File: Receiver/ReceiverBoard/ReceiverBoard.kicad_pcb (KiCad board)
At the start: 2 copper layers, 100 x 120 mm, 50 parts, among them IC1 SN74HCT245PWR, IC2 SN74HCT245PWR, J1 Left Header, J10 Output 5, J11 Output 6, J12 Output 7, J13 High Power, J14 Output 8, J15 Output 9, J16 Output 10, J17 Output 11, J18 Output 12, J19 Output 13, J2 Right Header, J20 Output 14, J21 Output 15, J22 J1B1211CCD, J3 Upper Middle Header, J4 Lower Middle Header, J5 Output 0, J6 Output 1, J7 Output 2, J8 Output 3, J9 Output 4

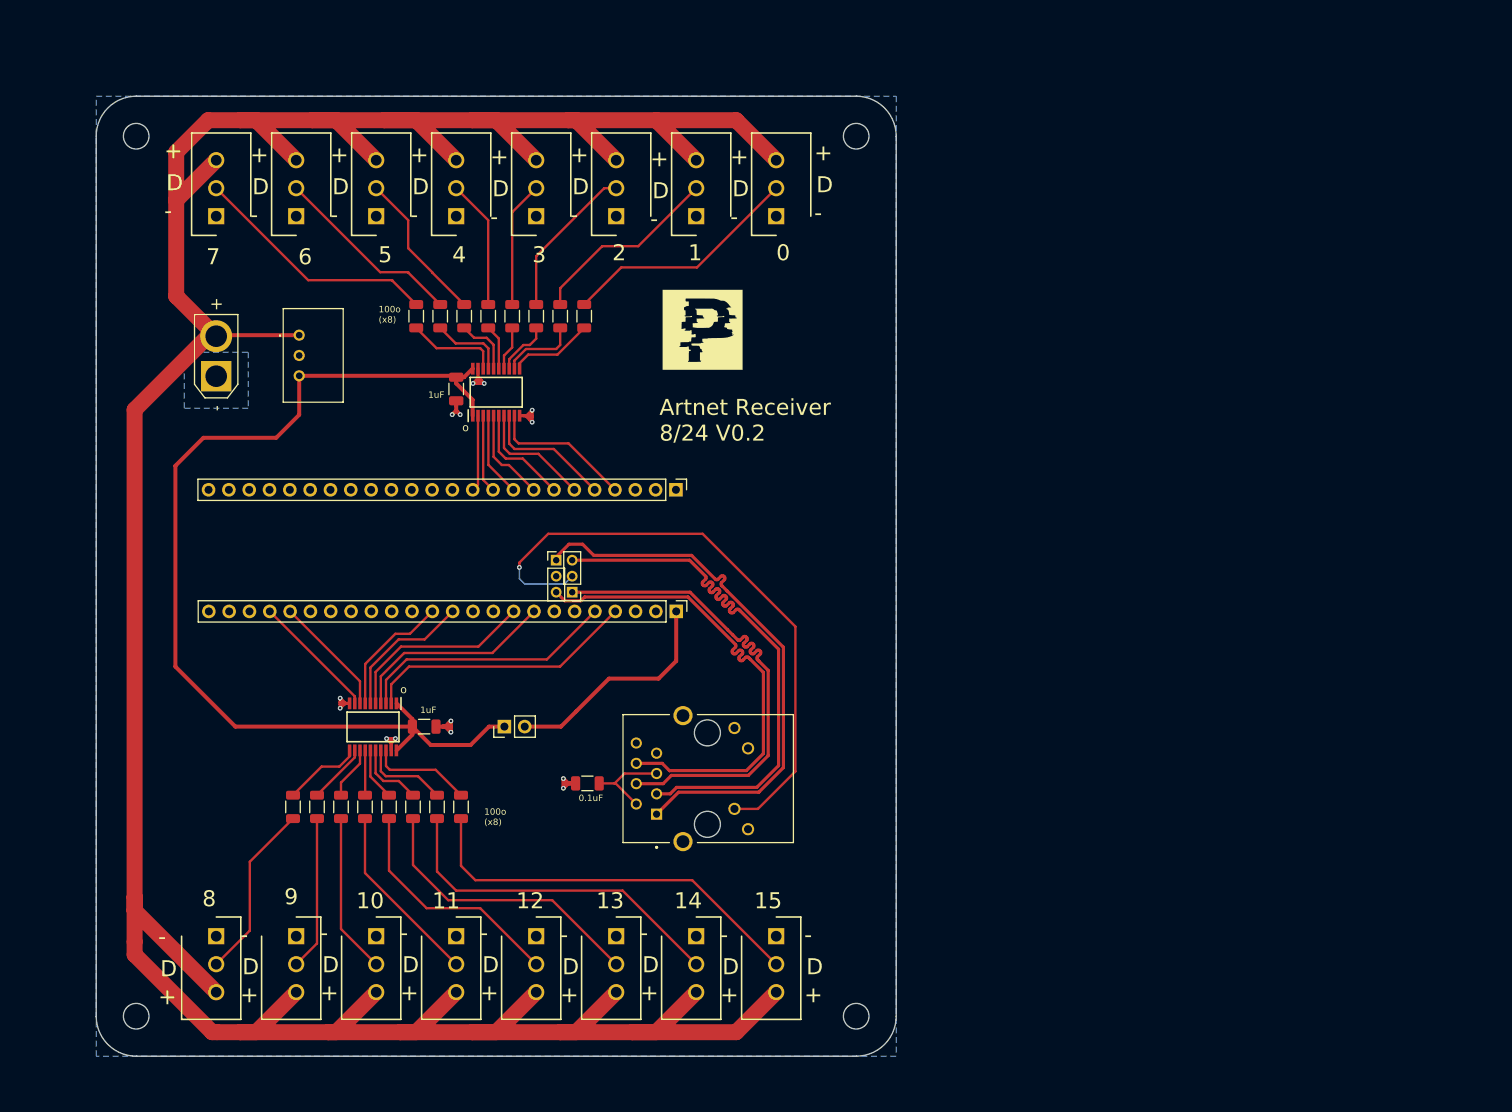
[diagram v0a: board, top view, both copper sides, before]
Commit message: Artnet is up and running!
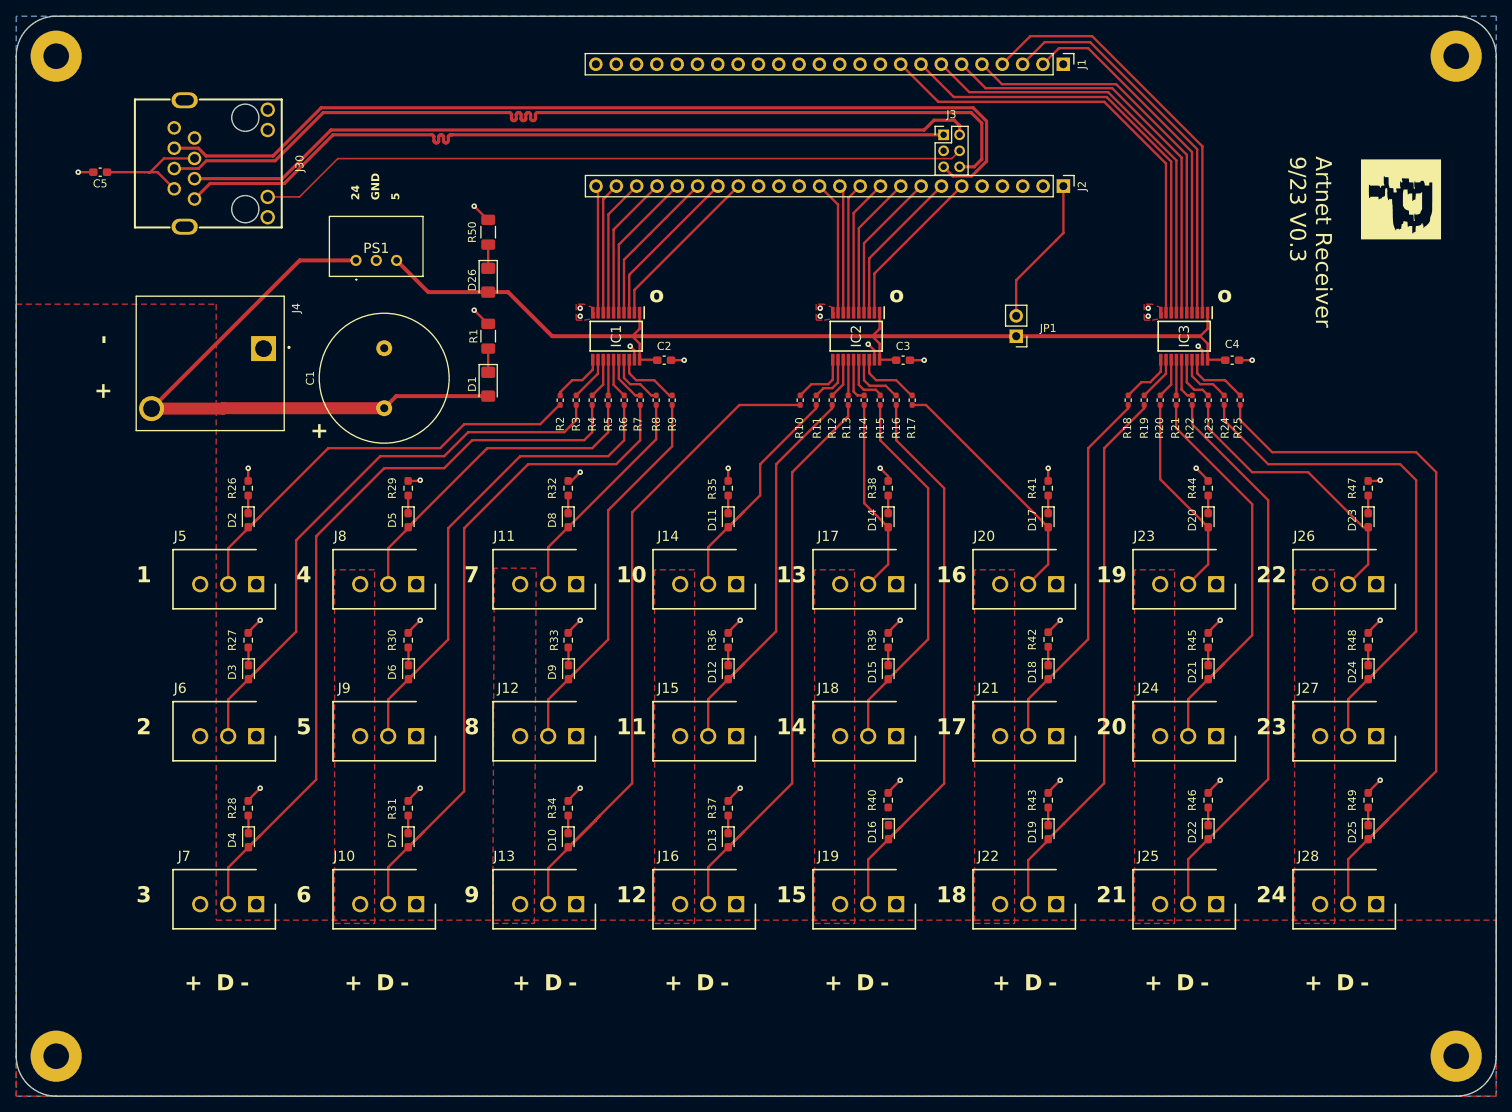
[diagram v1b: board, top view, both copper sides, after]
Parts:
- added C4: 1u, Capacitor_SMD:C_0603_1608Metric_Pad1.08x0.95mm_HandSolder, F.Cu at (217.0, 68.0)
- added C5: 100n, Capacitor_SMD:C_0603_1608Metric_Pad1.08x0.95mm_HandSolder, F.Cu at (75.5, 44.5)
- added D1: RED, LED_SMD:LED_1206_3216Metric_Pad1.42x1.75mm_HandSolder, F.Cu at (124.0, 71.0)
- added D10: YELLOW, LED_SMD:LED_0603_1608Metric_Pad1.05x0.95mm_HandSolder, F.Cu at (134.0, 128.0)
- added D11: YELLOW, LED_SMD:LED_0603_1608Metric_Pad1.05x0.95mm_HandSolder, F.Cu at (154.0, 88.0)
- added D12: YELLOW, LED_SMD:LED_0603_1608Metric_Pad1.05x0.95mm_HandSolder, F.Cu at (154.0, 107.0)
- added D13: YELLOW, LED_SMD:LED_0603_1608Metric_Pad1.05x0.95mm_HandSolder, F.Cu at (154.0, 128.0)
- added D14: YELLOW, LED_SMD:LED_0603_1608Metric_Pad1.05x0.95mm_HandSolder, F.Cu at (174.0, 88.0)
- added D15: YELLOW, LED_SMD:LED_0603_1608Metric_Pad1.05x0.95mm_HandSolder, F.Cu at (174.0, 107.0)
- added D16: YELLOW, LED_SMD:LED_0603_1608Metric_Pad1.05x0.95mm_HandSolder, F.Cu at (174.0, 127.0)
- added D17: YELLOW, LED_SMD:LED_0603_1608Metric_Pad1.05x0.95mm_HandSolder, F.Cu at (194.0, 88.0)
- added D18: YELLOW, LED_SMD:LED_0603_1608Metric_Pad1.05x0.95mm_HandSolder, F.Cu at (194.0, 107.0)
- added D19: YELLOW, LED_SMD:LED_0603_1608Metric_Pad1.05x0.95mm_HandSolder, F.Cu at (194.0, 127.0)
- added D2: YELLOW, LED_SMD:LED_0603_1608Metric_Pad1.05x0.95mm_HandSolder, F.Cu at (94.0, 88.0)
- added D20: YELLOW, LED_SMD:LED_0603_1608Metric_Pad1.05x0.95mm_HandSolder, F.Cu at (214.0, 88.0)
- added D21: YELLOW, LED_SMD:LED_0603_1608Metric_Pad1.05x0.95mm_HandSolder, F.Cu at (214.0, 107.0)
- added D22: YELLOW, LED_SMD:LED_0603_1608Metric_Pad1.05x0.95mm_HandSolder, F.Cu at (214.0, 127.0)
- added D23: YELLOW, LED_SMD:LED_0603_1608Metric_Pad1.05x0.95mm_HandSolder, F.Cu at (234.0, 88.0)
- added D24: YELLOW, LED_SMD:LED_0603_1608Metric_Pad1.05x0.95mm_HandSolder, F.Cu at (234.0, 107.0)
- added D25: YELLOW, LED_SMD:LED_0603_1608Metric_Pad1.05x0.95mm_HandSolder, F.Cu at (234.0, 127.0)
- added D26: RED, LED_SMD:LED_1206_3216Metric_Pad1.42x1.75mm_HandSolder, F.Cu at (124.0, 58.0)
- added D3: YELLOW, LED_SMD:LED_0603_1608Metric_Pad1.05x0.95mm_HandSolder, F.Cu at (94.0, 107.0)
- added D4: YELLOW, LED_SMD:LED_0603_1608Metric_Pad1.05x0.95mm_HandSolder, F.Cu at (94.0, 128.0)
- added D5: YELLOW, LED_SMD:LED_0603_1608Metric_Pad1.05x0.95mm_HandSolder, F.Cu at (114.0, 88.0)
- added D6: YELLOW, LED_SMD:LED_0603_1608Metric_Pad1.05x0.95mm_HandSolder, F.Cu at (114.0, 107.0)
- added D7: YELLOW, LED_SMD:LED_0603_1608Metric_Pad1.05x0.95mm_HandSolder, F.Cu at (114.0, 128.0)
- added D8: YELLOW, LED_SMD:LED_0603_1608Metric_Pad1.05x0.95mm_HandSolder, F.Cu at (134.0, 88.0)
- added D9: YELLOW, LED_SMD:LED_0603_1608Metric_Pad1.05x0.95mm_HandSolder, F.Cu at (134.0, 107.0)
- added IC3: SN74HCT245PWR, SN74HCT245PWR:SOP65P640X120-20N, F.Cu at (211.0, 65.0)
- added J23: String, 284514-3:SHDR3W80P0X350_1X3_1250X725X940P, F.Cu at (215.0, 96.0)
- added J24: String, 284514-3:SHDR3W80P0X350_1X3_1250X725X940P, F.Cu at (215.0, 115.0)
- added J25: String, 284514-3:SHDR3W80P0X350_1X3_1250X725X940P, F.Cu at (215.0, 136.0)
- added J26: String, 284514-3:SHDR3W80P0X350_1X3_1250X725X940P, F.Cu at (235.0, 96.0)
- added J27: String, 284514-3:SHDR3W80P0X350_1X3_1250X725X940P, F.Cu at (235.0, 115.0)
- added J28: String, 284514-3:SHDR3W80P0X350_1X3_1250X725X940P, F.Cu at (235.0, 136.0)
- added J30: RVB-ZZ-0004, RVB-ZZ-0004:RJ45-TH_RVB-ZZ-0004, F.Cu at (90.6, 43.4)
- added R17: 100, Resistor_SMD:R_0402_1005Metric_Pad0.72x0.64mm_HandSolder, F.Cu at (177.0, 73.0)
- added R18: 100, Resistor_SMD:R_0402_1005Metric_Pad0.72x0.64mm_HandSolder, F.Cu at (204.0, 73.0)
- added R19: 100, Resistor_SMD:R_0402_1005Metric_Pad0.72x0.64mm_HandSolder, F.Cu at (206.0, 73.0)
- added R20: 100, Resistor_SMD:R_0402_1005Metric_Pad0.72x0.64mm_HandSolder, F.Cu at (208.0, 73.0)
- added R21: 100, Resistor_SMD:R_0402_1005Metric_Pad0.72x0.64mm_HandSolder, F.Cu at (210.0, 73.0)
- added R22: 100, Resistor_SMD:R_0402_1005Metric_Pad0.72x0.64mm_HandSolder, F.Cu at (212.0, 73.0)
- added R23: 100, Resistor_SMD:R_0402_1005Metric_Pad0.72x0.64mm_HandSolder, F.Cu at (214.0, 73.0)
- added R24: 100, Resistor_SMD:R_0402_1005Metric_Pad0.72x0.64mm_HandSolder, F.Cu at (216.0, 73.0)
- added R25: 100, Resistor_SMD:R_0402_1005Metric_Pad0.72x0.64mm_HandSolder, F.Cu at (218.0, 73.0)
- added R26: 3k, Resistor_SMD:R_0603_1608Metric_Pad0.98x0.95mm_HandSolder, F.Cu at (94.0, 84.0)
- added R27: 3k, Resistor_SMD:R_0603_1608Metric_Pad0.98x0.95mm_HandSolder, F.Cu at (94.0, 103.0)
- added R28: 3k, Resistor_SMD:R_0603_1608Metric_Pad0.98x0.95mm_HandSolder, F.Cu at (94.0, 124.0)
- added R29: 3k, Resistor_SMD:R_0603_1608Metric_Pad0.98x0.95mm_HandSolder, F.Cu at (114.0, 84.0)
- added R30: 3k, Resistor_SMD:R_0603_1608Metric_Pad0.98x0.95mm_HandSolder, F.Cu at (114.0, 103.0)
- added R31: 3k, Resistor_SMD:R_0603_1608Metric_Pad0.98x0.95mm_HandSolder, F.Cu at (114.0, 124.0)
- added R32: 3k, Resistor_SMD:R_0603_1608Metric_Pad0.98x0.95mm_HandSolder, F.Cu at (134.0, 84.0)
- added R33: 3k, Resistor_SMD:R_0603_1608Metric_Pad0.98x0.95mm_HandSolder, F.Cu at (134.0, 103.0)
- added R34: 3k, Resistor_SMD:R_0603_1608Metric_Pad0.98x0.95mm_HandSolder, F.Cu at (134.0, 124.0)
- added R35: 3k, Resistor_SMD:R_0603_1608Metric_Pad0.98x0.95mm_HandSolder, F.Cu at (154.0, 84.0)
- added R36: 3k, Resistor_SMD:R_0603_1608Metric_Pad0.98x0.95mm_HandSolder, F.Cu at (154.0, 103.0)
- added R37: 3k, Resistor_SMD:R_0603_1608Metric_Pad0.98x0.95mm_HandSolder, F.Cu at (154.0, 124.0)
- added R38: 3k, Resistor_SMD:R_0603_1608Metric_Pad0.98x0.95mm_HandSolder, F.Cu at (174.0, 84.0)
- added R39: 3k, Resistor_SMD:R_0603_1608Metric_Pad0.98x0.95mm_HandSolder, F.Cu at (174.0, 103.0)
- added R40: 3k, Resistor_SMD:R_0603_1608Metric_Pad0.98x0.95mm_HandSolder, F.Cu at (174.0, 123.0)
- added R41: 3k, Resistor_SMD:R_0603_1608Metric_Pad0.98x0.95mm_HandSolder, F.Cu at (194.0, 84.0)
- added R42: 3k, Resistor_SMD:R_0603_1608Metric_Pad0.98x0.95mm_HandSolder, F.Cu at (194.0, 102.9)
- added R43: 3k, Resistor_SMD:R_0603_1608Metric_Pad0.98x0.95mm_HandSolder, F.Cu at (194.0, 123.0)
- added R44: 3k, Resistor_SMD:R_0603_1608Metric_Pad0.98x0.95mm_HandSolder, F.Cu at (214.0, 84.0)
- added R45: 3k, Resistor_SMD:R_0603_1608Metric_Pad0.98x0.95mm_HandSolder, F.Cu at (214.0, 103.0)
- added R46: 3k, Resistor_SMD:R_0603_1608Metric_Pad0.98x0.95mm_HandSolder, F.Cu at (214.0, 123.0)
- added R47: 3k, Resistor_SMD:R_0603_1608Metric_Pad0.98x0.95mm_HandSolder, F.Cu at (234.0, 84.0)
- added R48: 3k, Resistor_SMD:R_0603_1608Metric_Pad0.98x0.95mm_HandSolder, F.Cu at (234.0, 103.0)
- added R49: 3k, Resistor_SMD:R_0603_1608Metric_Pad0.98x0.95mm_HandSolder, F.Cu at (234.0, 123.0)
- added R50: 3.2k, Resistor_SMD:R_1206_3216Metric_Pad1.30x1.75mm_HandSolder, F.Cu at (124.0, 52.0)
- C1: value 1uF -> 1000u; footprint Capacitor_SMD:C_1206_3216Metric -> Capacitor_THT:C_Radial_D16.0mm_H25.0mm_P7.50mm
- C2: value 1uF -> 1u; footprint Capacitor_SMD:C_1206_3216Metric -> Capacitor_SMD:C_0603_1608Metric_Pad1.08x0.95mm_HandSolder
- C3: value 0.1uF -> 1u; footprint Capacitor_SMD:C_1206_3216Metric -> Capacitor_SMD:C_0603_1608Metric_Pad1.08x0.95mm_HandSolder
- H1, H2, H3, H4: footprint MountingHole:MountingHole_3.2mm_M3 -> MountingHole:MountingHole_3.2mm_M3_Pad
- J10: value Output 5 -> String
- J11: value Output 6 -> String
- J12: value Output 7 -> String
- J13: value High Power -> String; footprint Connector_AMASS:AMASS_XT30U-F_1x02_P5.0mm_Vertical -> 284514-3:SHDR3W80P0X350_1X3_1250X725X940P
- J14: value Output 8 -> String
- J15: value Output 9 -> String
- J16: value Output 10 -> String
- J17: value Output 11 -> String
- J18: value Output 12 -> String
- J19: value Output 13 -> String
- J20: value Output 14 -> String
- J21: value Output 15 -> String
- J22: value J1B1211CCD -> String; footprint J1B1211CCD:J1B1211CCD -> 284514-3:SHDR3W80P0X350_1X3_1250X725X940P
- J3: value Upper Middle Header -> Ethernet; footprint Connector_PinHeader_2.00mm:PinHeader_1x03_P2.00mm_Vertical -> Connector_PinHeader_2.00mm:PinHeader_2x03_P2.00mm_Vertical
- J4: value Lower Middle Header -> 1719312; footprint Connector_PinHeader_2.00mm:PinHeader_1x03_P2.00mm_Vertical -> 1719312:PHOENIX_1719312
- J5: value Output 0 -> String
- J6: value Output 1 -> String
- J7: value Output 2 -> String
- J8: value Output 3 -> String
- J9: value Output 4 -> String
- PS1: footprint KiCad:TSR12450E -> TSR_1-2450E:TSR12450E
- R1: value 100 -> 3.3k; footprint Resistor_SMD:R_1206_3216Metric -> Resistor_SMD:R_1206_3216Metric_Pad1.30x1.75mm_HandSolder
- R10, R11, R12, R13, R14, R15, R2, R3, R4, R5, R6, R7, R9: footprint Resistor_SMD:R_1206_3216Metric -> Resistor_SMD:R_0402_1005Metric_Pad0.72x0.64mm_HandSolder
- R16, R8: value 100(x8) -> 100; footprint Resistor_SMD:R_1206_3216Metric -> Resistor_SMD:R_0402_1005Metric_Pad0.72x0.64mm_HandSolder
- moved J7 97.1 mm to (95.0, 136.0), turned to 180 degrees
- moved R16 90.9 mm to (175.0, 73.0)
- moved G*** 88.8 mm to (238.1, 47.9), turned to -90 degrees
- moved R15 86.8 mm to (173.0, 73.0)
- moved J10 86.1 mm to (115.0, 136.0), turned to 180 degrees
- moved J6 85.1 mm to (95.0, 115.0), turned to 180 degrees
- moved R14 82.8 mm to (171.0, 73.0)
- moved JP1 80.5 mm to (190.0, 65.0), turned to 180 degrees
- moved J13 79.9 mm to (135.0, 136.0), turned to 180 degrees
- moved J5 79.6 mm to (95.0, 96.0), turned to 180 degrees
- moved J12 79.1 mm to (135.0, 115.0), turned to 180 degrees
- moved R13 78.9 mm to (169.0, 73.0)
- moved J14 78.5 mm to (155.0, 96.0), turned to 180 degrees
- moved IC2 77.7 mm to (170.0, 65.0)
- moved H2 75.7 mm to (245.0, 30.0)
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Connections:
- C1 pad 1: GND -> +24V
- C1 pad 2: +5V -> GND
- C3 pad 1: Net-(J22-RCT) -> GND
- C3 pad 2: GND -> +5V
- IC1 pad 2: D7 -> D8
- IC1 pad 3: D6 -> D7
- IC1 pad 4: D5 -> D6
- IC1 pad 5: D4 -> D5
- IC1 pad 6: D3 -> D4
- IC1 pad 7: D2 -> D3
- IC1 pad 8: D1 -> D2
- IC1 pad 9: D0 -> D1
- IC2 pad 2: D15 -> D16
- IC2 pad 3: D14 -> D15
- IC2 pad 4: D13 -> D14
- IC2 pad 5: D12 -> D13
- IC2 pad 6: D11 -> D12
- IC2 pad 7: D10 -> D11
- IC2 pad 8: D9 -> D10
- IC2 pad 9: D8 -> D9
- J1 pad 10: D6 -> unconnected-(J1-Pin_10-Pad10)
- J1 pad 11: D7 -> unconnected-(J1-Pin_11-Pad11)
- J1 pad 2: unconnected-(J1-Pin_2-Pad2) -> D22
- J1 pad 3: unconnected-(J1-Pin_3-Pad3) -> D23
- J1 pad 4: D0 -> D24
- J1 pad 5: D1 -> D21
- J1 pad 6: D2 -> D20
- J1 pad 7: D3 -> D19
- J1 pad 8: D4 -> D18
- J1 pad 9: D5 -> D17
- J10 pad 2: D5O -> D6O
- J11 pad 2: D6O -> D7O
- J12 pad 2: D7O -> D8O
- J13 pad 2: +24V -> D9O
- J14 pad 2: D8O -> D10O
- J15 pad 2: D9O -> D11O
- J16 pad 2: D10O -> D12O
- J17 pad 2: D11O -> D13O
- J18 pad 2: D12O -> D14O
- J19 pad 2: D13O -> D15O
- J2 pad 10: unconnected-(J2-Pin_10-Pad10) -> D12
- J2 pad 11: unconnected-(J2-Pin_11-Pad11) -> D11
- J2 pad 12: D11 -> D10
- J2 pad 13: D10 -> D9
- J2 pad 17: unconnected-(J2-Pin_17-Pad17) -> D8
- J2 pad 18: unconnected-(J2-Pin_18-Pad18) -> D7
- J2 pad 19: unconnected-(J2-Pin_19-Pad19) -> D6
- J2 pad 20: D9 -> D5
- J2 pad 21: D8 -> D4
- J2 pad 22: unconnected-(J2-Pin_22-Pad22) -> D3
- J2 pad 23: unconnected-(J2-Pin_23-Pad23) -> D2
- J2 pad 24: unconnected-(J2-Pin_24-Pad24) -> D1
- J2 pad 4: D15 -> unconnected-(J2-Pin_4-Pad4)
- J2 pad 5: D14 -> unconnected-(J2-Pin_5-Pad5)
- J2 pad 6: unconnected-(J2-Pin_6-Pad6) -> D16
- J2 pad 7: unconnected-(J2-Pin_7-Pad7) -> D15
- J2 pad 8: D13 -> D14
- J2 pad 9: D12 -> D13
- J20 pad 2: D14O -> D16O
- J21 pad 2: D15O -> D17O
- J22 pad 1: TX+ -> GND
- J22 pad 2: Net-(J22-RCT) -> D18O
- J22 pad 3: TX- -> +24V
- J3 pad 1: RX+ -> TX+
- J3 pad 2: ELED -> TX-
- J3 pad 3: TX- -> GND
- J4 pad 1: TX+ -> GND
- J4 pad 2: GND -> +24V
- J5 pad 2: D0O -> D1O
- J6 pad 2: D1O -> D2O
- J7 pad 2: D2O -> D3O
- J8 pad 2: D3O -> D4O
- J9 pad 2: D4O -> D5O
- R1 pad 1: Net-(IC1-B1) -> Net-(D1-K)
- R1 pad 2: D7O -> GND
- R10 pad 1: Net-(IC2-B2) -> D9O
- R10 pad 2: D14O -> Net-(IC2-B8)
- R11 pad 1: Net-(IC2-B3) -> Net-(IC2-B7)
- R11 pad 2: D13O -> D10O
- R12 pad 1: Net-(IC2-B4) -> Net-(IC2-B6)
- R12 pad 2: D12O -> D11O
- R13 pad 2: D11O -> D12O
- R14 pad 1: Net-(IC2-B6) -> Net-(IC2-B4)
- R14 pad 2: D10O -> D13O
- R15 pad 1: Net-(IC2-B7) -> Net-(IC2-B3)
- R15 pad 2: D9O -> D14O
- R16 pad 1: Net-(IC2-B8) -> Net-(IC2-B2)
- R16 pad 2: D8O -> D15O
- R2 pad 1: Net-(IC1-B2) -> D1O
- R2 pad 2: D6O -> Net-(IC1-B8)
- R3 pad 1: Net-(IC1-B3) -> Net-(IC1-B7)
- R3 pad 2: D5O -> D2O
- R4 pad 1: Net-(IC1-B4) -> Net-(IC1-B6)
- R4 pad 2: D4O -> D3O
- R5 pad 2: D3O -> D4O
- R6 pad 1: Net-(IC1-B6) -> Net-(IC1-B4)
- R6 pad 2: D2O -> D5O
- R7 pad 1: Net-(IC1-B7) -> Net-(IC1-B3)
- R7 pad 2: D1O -> D6O
- R8 pad 1: Net-(IC1-B8) -> Net-(IC1-B2)
- R8 pad 2: D0O -> D7O
- R9 pad 1: Net-(IC2-B1) -> Net-(IC1-B1)
- R9 pad 2: D15O -> D8O
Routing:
- net +24V: track 416.7 -> 76.6 mm
- net D24O: track 0.00 -> 91.1 mm
- net D3O: track 15.8 -> 95.8 mm
- net D21O: track 0.00 -> 70.5 mm
- net D18O: track 0.00 -> 68.4 mm
- net D9O: track 19.3 -> 85.5 mm
- net D23O: track 0.00 -> 65.9 mm
- net D6O: track 24.0 -> 84.6 mm
- net D17: track 0.00 -> 56.9 mm
- net RX-: track 60.8 -> 116.8 mm
- net D18: track 0.00 -> 55.2 mm
- net RX+: track 61.8 -> 116.7 mm
- net D2O: track 19.6 -> 74.2 mm
- net D19: track 0.00 -> 53.4 mm
- net D24: track 0.00 -> 53.0 mm
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- added copper zone on F.Cu, net +24V
- added copper zone on F.Cu, net GND
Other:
- board size 100 x 120 mm -> 185 x 135 mm
- board text added: "16"
- board text added: "17"
- board text added: "18"
- board text added: "19"
- board text added: "20"
- board text added: "21"
- board text added: "22"
- board text added: "23"
- board text added: "24"
- board text added: "Artnet Receiver 9/23 V0.3"
- board text added: "GND"
- board text removed: "0"
- board text removed: "0.1uF"
- board text removed: "100o (x8)"
- board text removed: "1uF"
- board text removed: "Artnet Receiver 8/24 V0.2"
